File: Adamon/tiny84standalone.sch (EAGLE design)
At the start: 28 parts

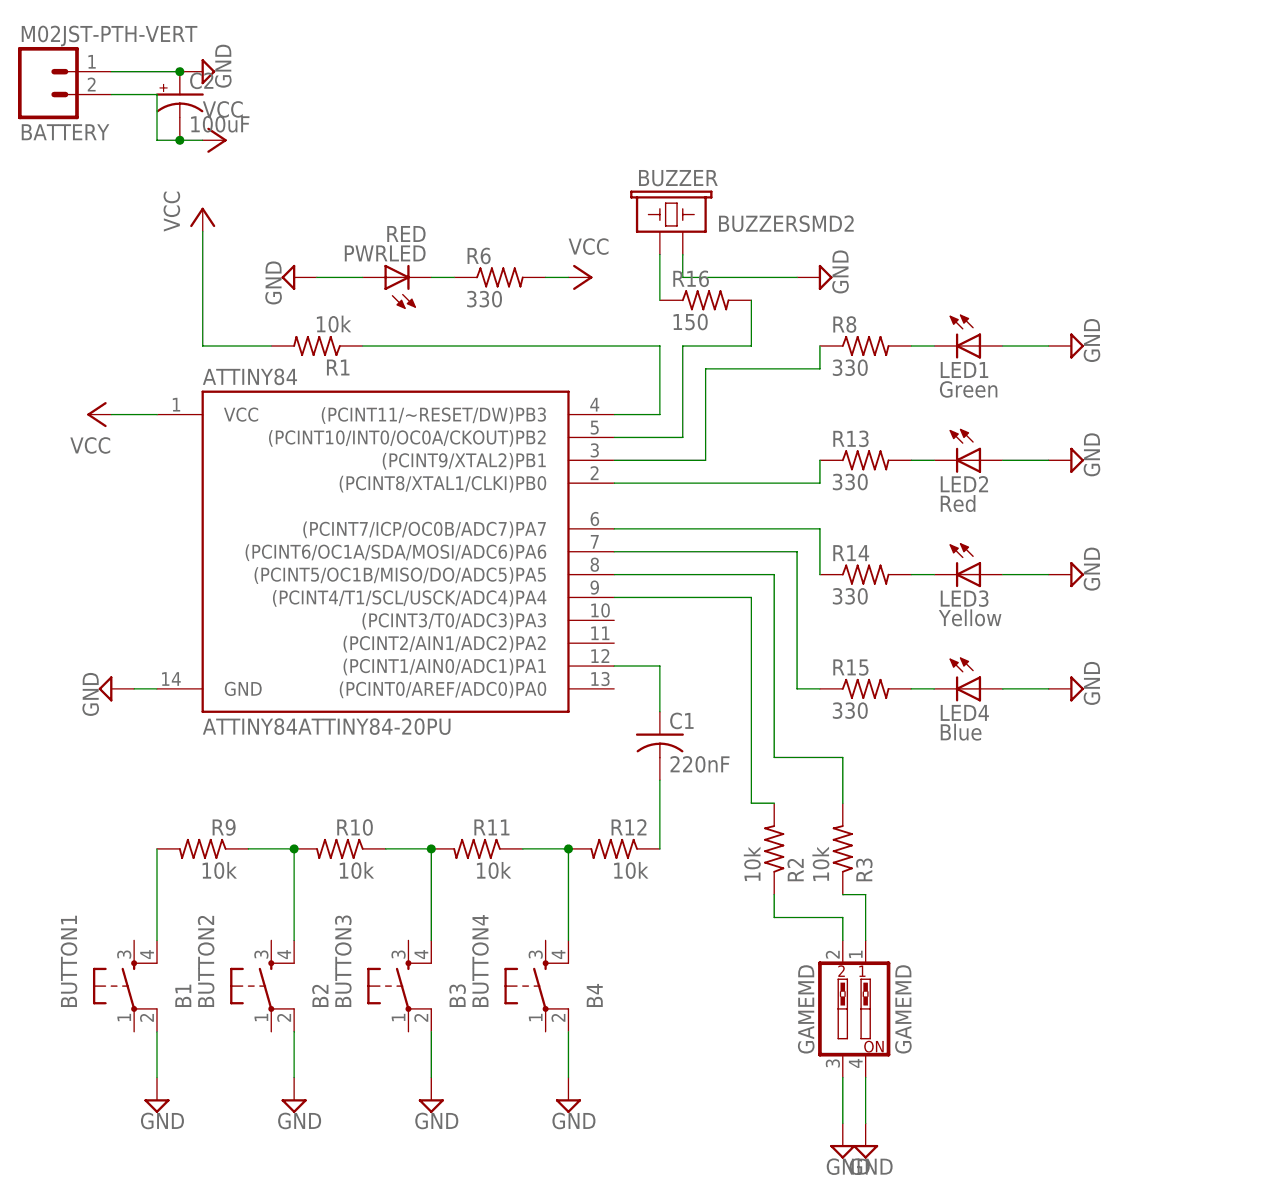
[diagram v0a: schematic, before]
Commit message: better schematic
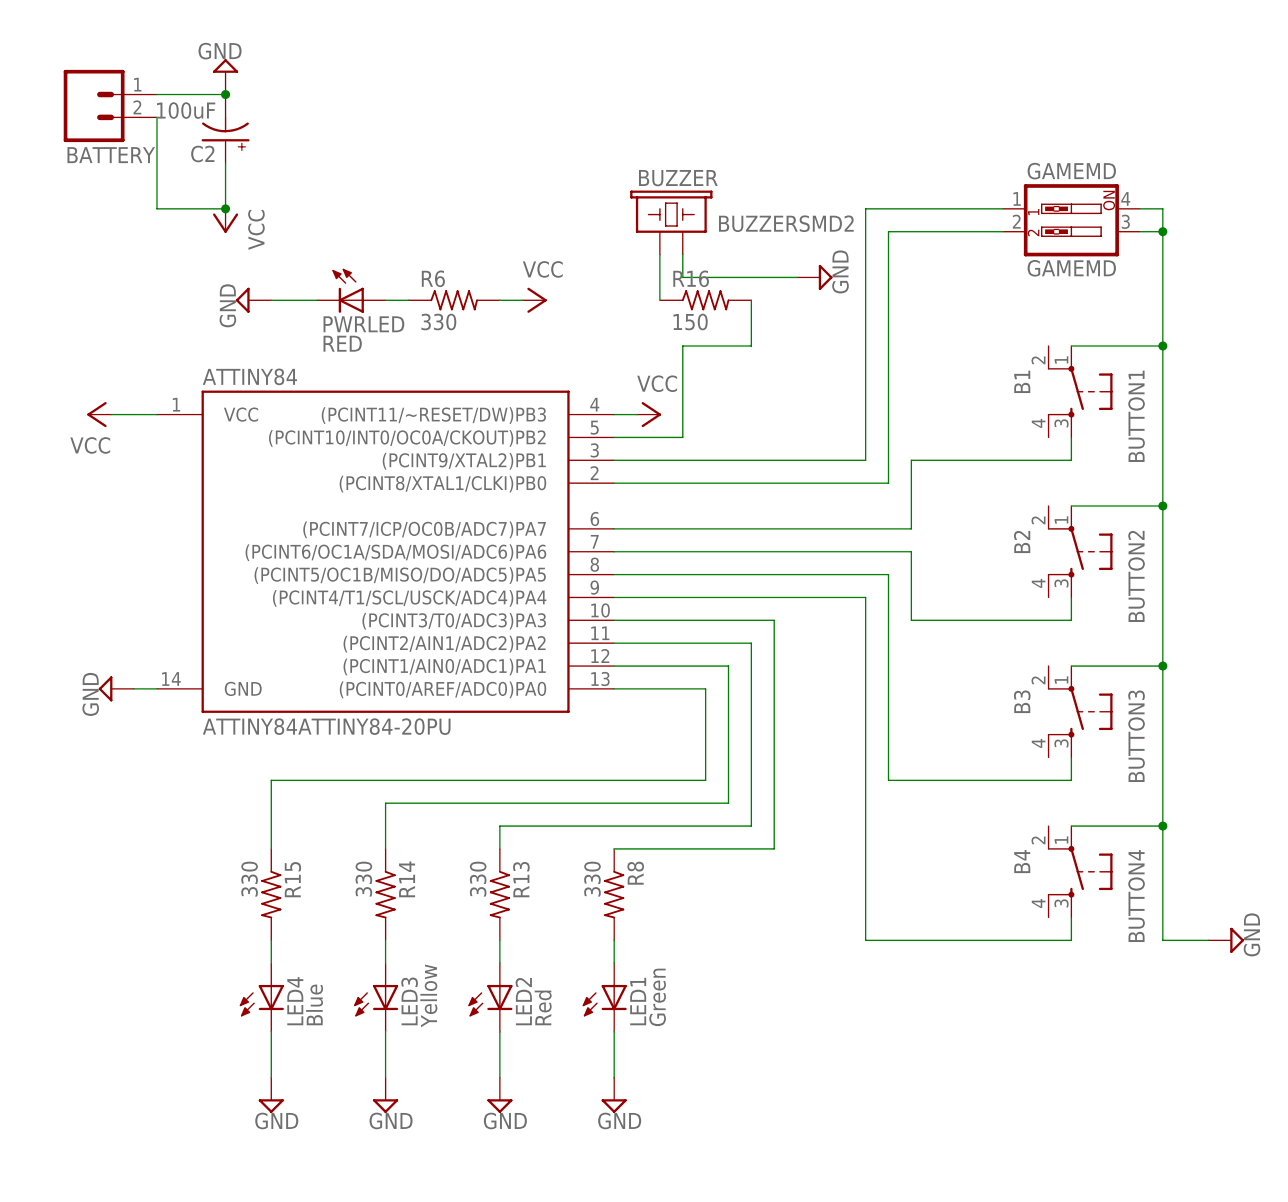
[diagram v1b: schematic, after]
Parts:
- removed C1: 220nF, resistor:C-USC0805
- removed R1: 10k, resistor:R-US_R0805
- removed R10, R11, R12, R2, R3, R9: 10k, rcl:R-US_R0805
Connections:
- removed net N$12: ATTINY84.(PCINT7/ICP/OC0B/ADC7)PA7, R14.1
- removed net N$19: ATTINY84.(PCINT5/OC1B/MISO/DO/ADC5)PA5, R3.2
- removed net N$20: BUTTON4.4, R11.1, R12.2
- removed net N$21: ATTINY84.(PCINT4/T1/SCL/USCK/ADC4)PA4, R2.2
- removed net N$22: ATTINY84.(PCINT1/AIN0/ADC1)PA1, C1.1
- removed net N$32: LED4.C, R15.2
- removed net N$33: LED3.C, R14.2
- removed net N$35: LED2.C, R13.2
- removed net N$37: LED1.C, R8.2
- new net N$2: PWRLED.A, R6.1
- new net N$3: LED1.A, R8.2
- new net N$7: LED3.A, R14.2
- new net N$8: LED4.A, R15.2
- net GND: now also BUTTON1.1, BUTTON2.1, BUTTON3.1, BUTTON4.1, C2.-, LED1.C, LED2.C, LED3.C, LED4.C, PWRLED.C; no longer BUTTON1.2, BUTTON2.2, BUTTON3.2, BUTTON4.2, C2.+, LED1.A, LED2.A, LED3.A, LED4.A, PWRLED.A
- net N$10: now also GAMEMD.1; no longer R8.1
- net N$11: now also GAMEMD.2; no longer R13.1
- net N$13: now also ATTINY84.(PCINT5/OC1B/MISO/DO/ADC5)PA5, BUTTON3.3; no longer ATTINY84.(PCINT6/OC1A/SDA/MOSI/ADC6)PA6, R15.1
- net N$14: now also ATTINY84.(PCINT4/T1/SCL/USCK/ADC4)PA4, BUTTON4.3; no longer BUTTON1.4, R9.2
- net N$15: now also ATTINY84.(PCINT3/T0/ADC3)PA3, R8.1; no longer GAMEMD.1, R3.1
- net N$16: now also ATTINY84.(PCINT2/AIN1/ADC2)PA2, R13.1; no longer GAMEMD.2, R2.1
- net N$17: now also ATTINY84.(PCINT1/AIN0/ADC1)PA1, R14.1; no longer BUTTON2.4, R10.2, R9.1
- net N$18: now also ATTINY84.(PCINT0/AREF/ADC0)PA0, R15.1; no longer BUTTON3.4, R10.1, R11.2
- net N$4: now also LED2.A, R13.2; no longer PWRLED.C, R6.1
- net N$5: now also ATTINY84.(PCINT7/ICP/OC0B/ADC7)PA7, BUTTON1.3; no longer ATTINY84.(PCINT11/~RESET/DW)PB3, R1.1
- net N$9: now also ATTINY84.(PCINT6/OC1A/SDA/MOSI/ADC6)PA6, BUTTON2.3; no longer C1.2, R12.1
- net VCC: now also ATTINY84.(PCINT11/~RESET/DW)PB3, C2.+; no longer C2.-, R1.2
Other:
- moved on the sheet: BATTERY, BUTTON1, BUTTON2, BUTTON3, BUTTON4, C2, GAMEMD, LED1, LED2, LED3, LED4, PWRLED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
